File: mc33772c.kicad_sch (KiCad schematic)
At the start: 11 parts, among them U2 MC33772CTP1AE

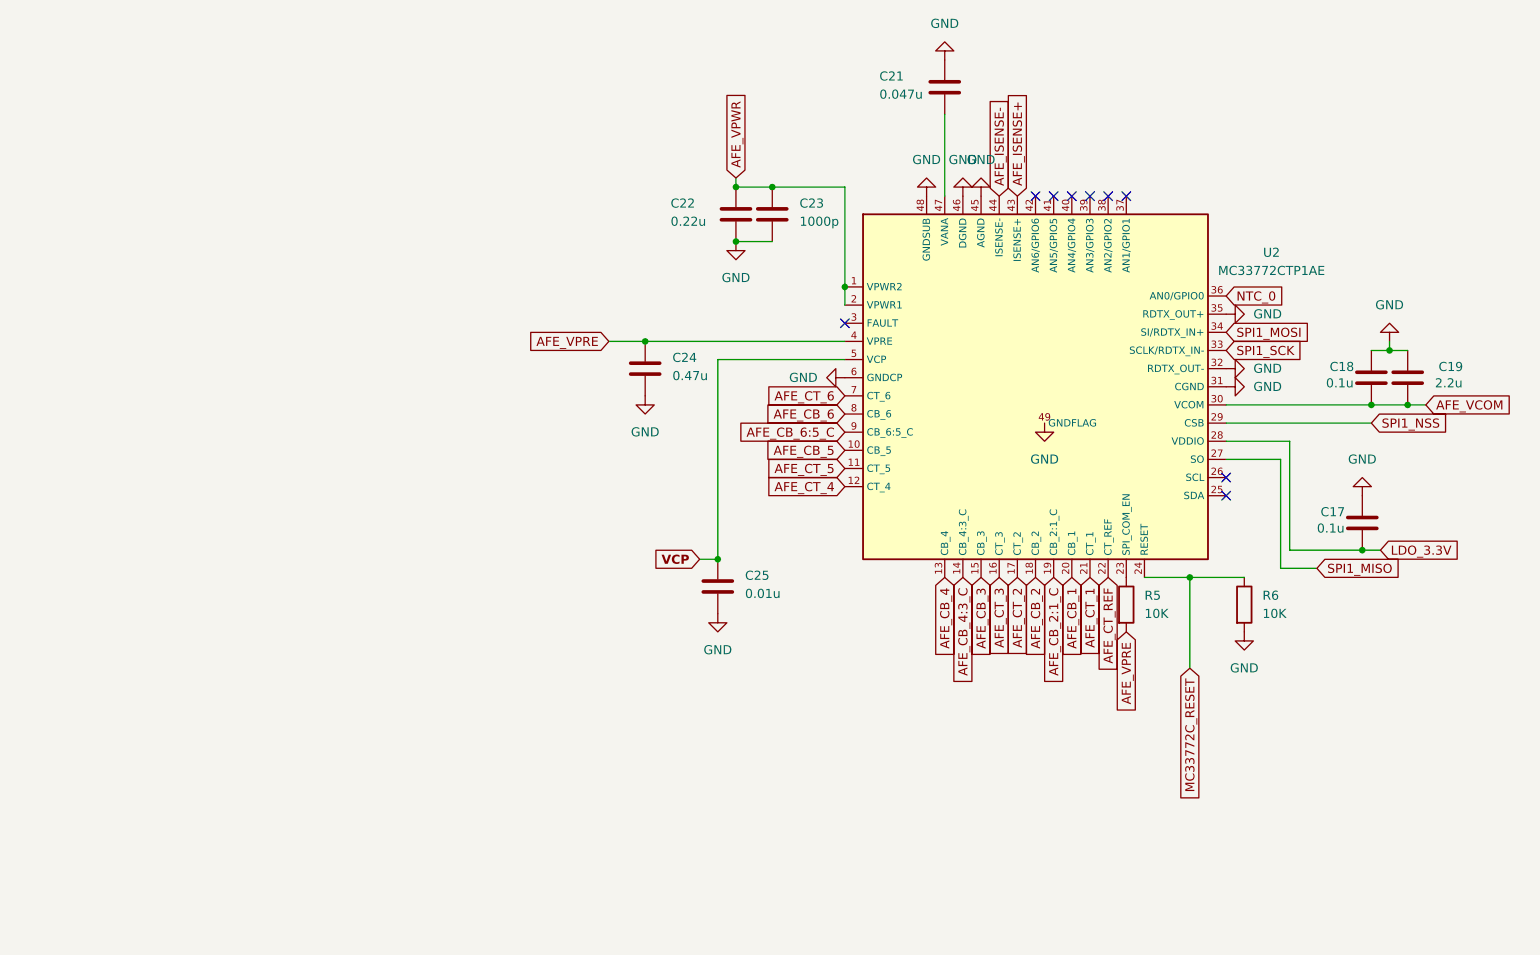
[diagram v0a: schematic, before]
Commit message: schematic done
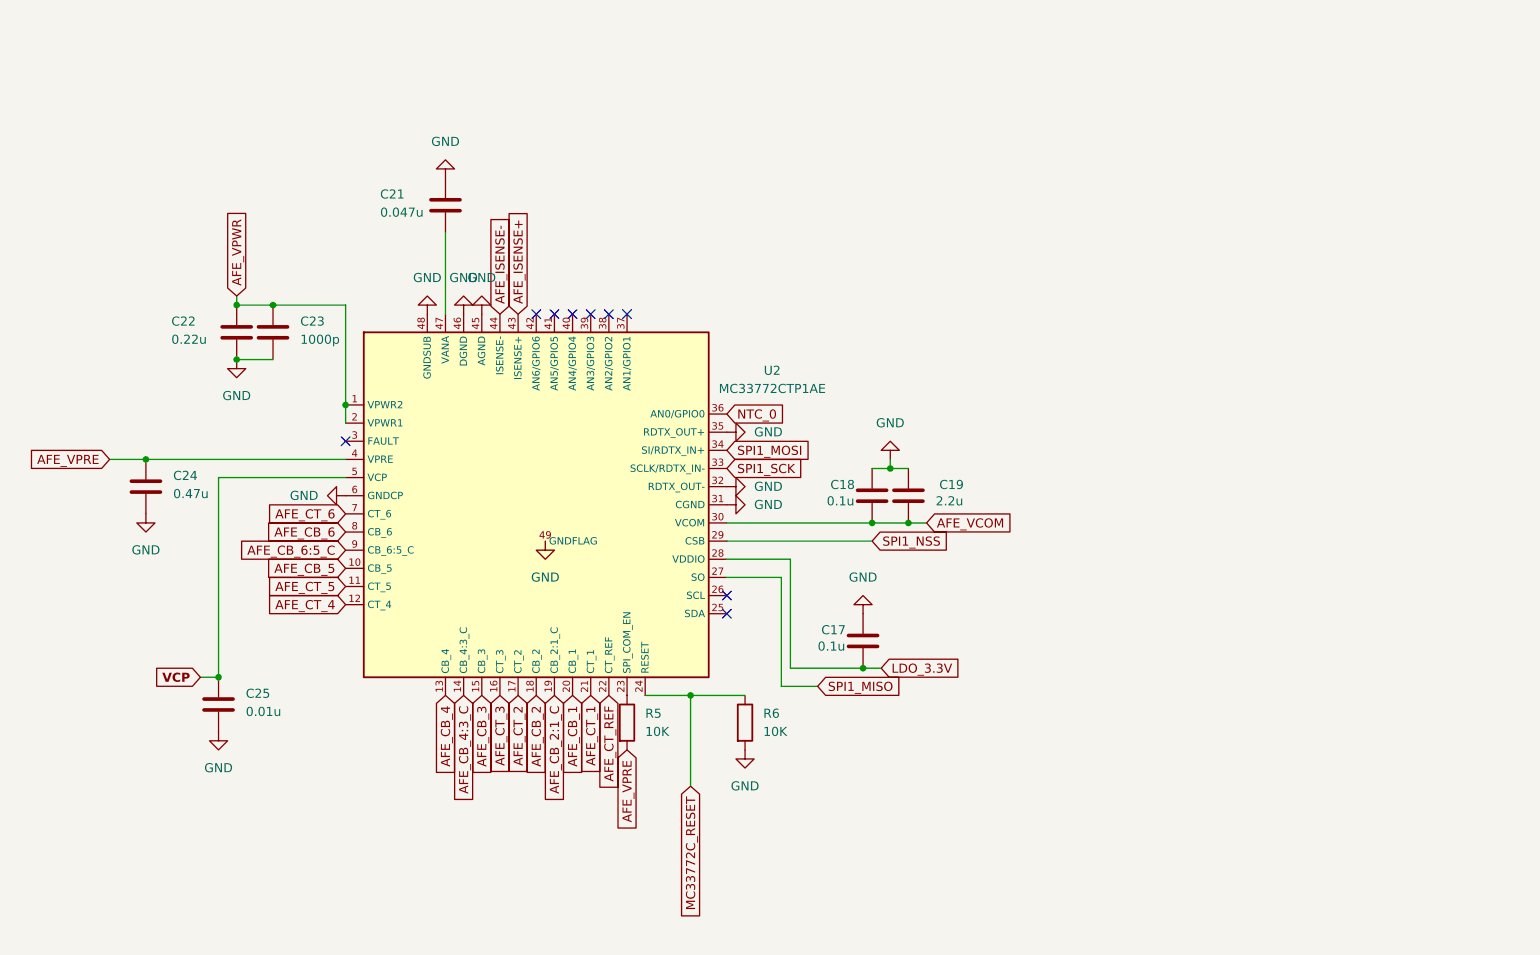
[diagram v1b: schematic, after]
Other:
- moved on the sheet: C17, C18, C19, C21, C22, C23, C24, C25, R5, R6, U2
